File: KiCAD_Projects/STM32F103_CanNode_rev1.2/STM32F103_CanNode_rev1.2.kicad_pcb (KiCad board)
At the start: 2 copper layers, 35 x 50 mm, 77 parts, among them P1 CONN_01X04, P10 CONN_01X04, P11 CONN_01X04, P12 CONN_01X02, P2 CONN_01X04, P3 CONN_01X08, P4 CONN_01X08, P5 CONN_01X06, P6 CONN_01X02, P7 CONN_01X08, P8 CONN_01X04, P9 CONN_01X04, SW1 SW_PUSH, SW2 SW_PUSH, U1 STM32F103_48, U2 AOZ1280, U3 MAX3051, U4 NCP1117ST50T3G, U5 TBD62083A, X2 CRYSTAL

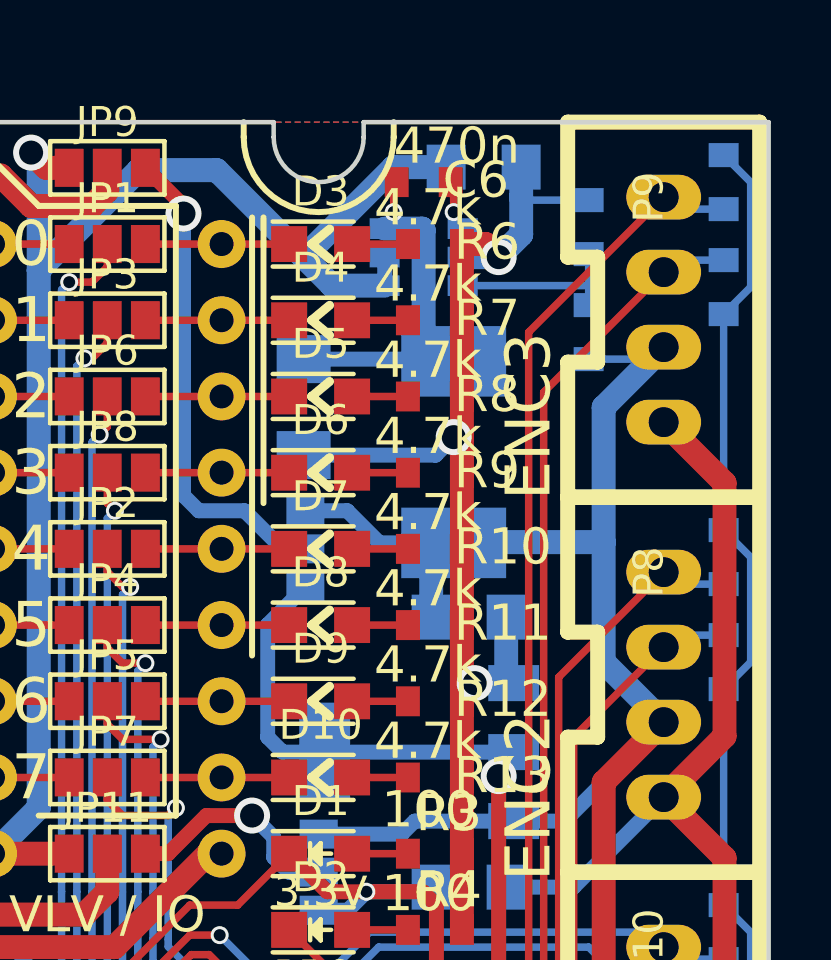
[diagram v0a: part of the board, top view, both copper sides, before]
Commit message: セルチェッカー作った｡電源基板ver1.1作った｡ぶっさしMDいじった｡DCDCいじりだした｡
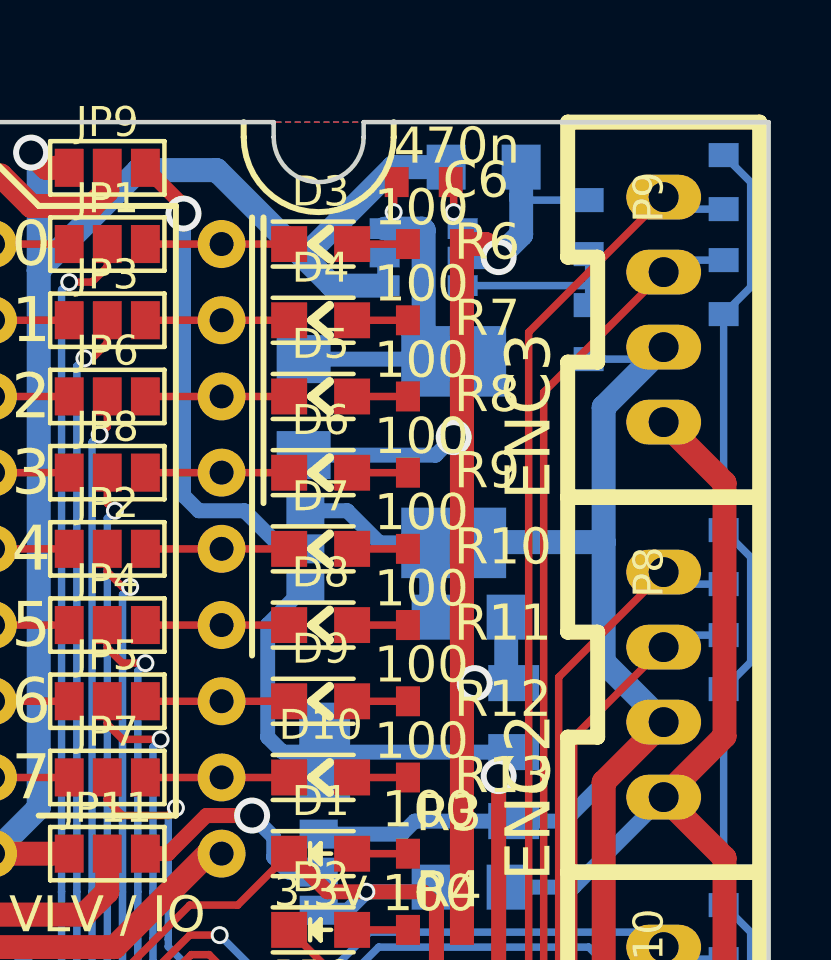
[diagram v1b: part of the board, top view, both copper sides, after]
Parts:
- R10, R11, R12, R13, R6, R7, R8, R9: value 4.7k -> 100
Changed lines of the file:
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@@
     (links 193)
     (no_connects 0)
-    (area -0.075001 -0.075001 35.075001 50.075001)
+    (area -3.509333 -2.533334 35.150001 52.533333)
     (thickness 1.6)
     (drawings 50)
@@
       (effects (font (size 1.2065 1.2065) (thickness 0.1016)) (justify left bottom))
     )
-    (fp_text value 4.7k (at 2.032 0.508 180) (layer F.SilkS)
+    (fp_text value 100 (at 2.032 0.508 180) (layer F.SilkS)
       (effects (font (size 1.2065 1.2065) (thickness 0.1016)) (justify left bottom))
     )
@@
       (effects (font (size 1.2065 1.2065) (thickness 0.1016)) (justify left bottom))
     )
-    (fp_text value 4.7k (at 2.032 0.508 180) (layer F.SilkS)
+    (fp_text value 100 (at 2.032 0.508 180) (layer F.SilkS)
       (effects (font (size 1.2065 1.2065) (thickness 0.1016)) (justify left bottom))
     )
@@
       (effects (font (size 1.2065 1.2065) (thickness 0.1016)) (justify left bottom))
     )
-    (fp_text value 4.7k (at 2.032 0.508 180) (layer F.SilkS)
+    (fp_text value 100 (at 2.032 0.508 180) (layer F.SilkS)
       (effects (font (size 1.2065 1.2065) (thickness 0.1016)) (justify left bottom))
     )
@@
       (effects (font (size 1.2065 1.2065) (thickness 0.1016)) (justify left bottom))
     )
-    (fp_text value 4.7k (at 2.032 0.508 180) (layer F.SilkS)
+    (fp_text value 100 (at 2.032 0.508 180) (layer F.SilkS)
       (effects (font (size 1.2065 1.2065) (thickness 0.1016)) (justify left bottom))
     )
@@
       (effects (font (size 1.2065 1.2065) (thickness 0.1016)) (justify left bottom))
     )
-    (fp_text value 4.7k (at 2.032 0.508 180) (layer F.SilkS)
+    (fp_text value 100 (at 2.032 0.508 180) (layer F.SilkS)
       (effects (font (size 1.2065 1.2065) (thickness 0.1016)) (justify left bottom))
     )
@@
       (effects (font (size 1.2065 1.2065) (thickness 0.1016)) (justify left bottom))
     )
-    (fp_text value 4.7k (at 2.032 0.508 180) (layer F.SilkS)
+    (fp_text value 100 (at 2.032 0.508 180) (layer F.SilkS)
       (effects (font (size 1.2065 1.2065) (thickness 0.1016)) (justify left bottom))
     )
@@
       (effects (font (size 1.2065 1.2065) (thickness 0.1016)) (justify left bottom))
     )
-    (fp_text value 4.7k (at 2.032 0.508 180) (layer F.SilkS)
+    (fp_text value 100 (at 2.032 0.508 180) (layer F.SilkS)
       (effects (font (size 1.2065 1.2065) (thickness 0.1016)) (justify left bottom))
     )
@@
       (effects (font (size 1.2065 1.2065) (thickness 0.1016)) (justify left bottom))
     )
-    (fp_text value 4.7k (at 2.032 0.508 180) (layer F.SilkS)
+    (fp_text value 100 (at 2.032 0.508 180) (layer F.SilkS)
       (effects (font (size 1.2065 1.2065) (thickness 0.1016)) (justify left bottom))
     )
@@
       (effects (font (size 1.2065 1.2065) (thickness 0.1016)) (justify left bottom mirror))
     )
-    (fp_text value 0.1u (at 0.88 -0.67) (layer B.SilkS)
+    (fp_text value 0.1u (at 2.88 4.33) (layer B.SilkS)
       (effects (font (size 1.2065 1.2065) (thickness 0.1016)) (justify left bottom mirror))
     )
@@
       (effects (font (size 1.2065 1.2065) (thickness 0.1016)) (justify left bottom mirror))
     )
-    (fp_text value 4.7k (at -1.5 1 270) (layer B.SilkS)
+    (fp_text value 4.7k (at -0.5 0.5 360) (layer B.SilkS)
       (effects (font (size 1.2065 1.2065) (thickness 0.1016)) (justify left bottom mirror))
     )
@@
       (effects (font (size 1.2065 1.2065) (thickness 0.1016)) (justify left bottom mirror))
     )
-    (fp_text value 4.7k (at -0.5 0.5 180) (layer B.SilkS)
+    (fp_text value 4.7k (at -1.5 1 270) (layer B.SilkS)
       (effects (font (size 1.2065 1.2065) (thickness 0.1016)) (justify left bottom mirror))
     )
@@
   (segment (start 10.668 4.932) (end 10.668 22.86) (width 0.8) (layer B.Cu) (net 3))
   (segment (start 11.684 24.384) (end 9.144 24.384) (width 0.8) (layer F.Cu) (net 3))
-  (segment (start 20.045584 38.356245) (end 21.5 39.810661) (width 0.25) (layer F.Cu) (net 4) (status 400000))
-  (segment (start 22.5 42.3) (end 22.5 44.3) (width 0.25) (layer B.Cu) (net 4) (status 800000))
+  (segment (start 20.045584 38.356245) (end 21.5 39.810661) (width 0.25) (layer F.Cu) (net 4))
+  (segment (start 22.5 42.3) (end 22.5 44.3) (width 0.25) (layer B.Cu) (net 4))
   (via (at 22.5 42.3) (size 0.6) (drill 0.4) (layers F.Cu B.Cu) (net 4))
   (segment (start 21.5 41.3) (end 22.5 42.3) (width 0.25) (layer F.Cu) (net 4))
@@
   (segment (start 22.3 44.5) (end 22.5 44.3) (width 0.25) (layer B.Cu) (net 4))
   (segment (start 22.2 45) (end 22.5 45.3) (width 0.25) (layer B.Cu) (net 4))
-  (segment (start 20.399138 38.002691) (end 22 39.603553) (width 0.25) (layer F.Cu) (net 5) (status 400000))
+  (segment (start 20.399138 38.002691) (end 22 39.603553) (width 0.25) (layer F.Cu) (net 5))
   (via (at 22.5 41) (size 0.6) (drill 0.4) (layers F.Cu B.Cu) (net 5))
   (segment (start 22 40.5) (end 22.5 41) (width 0.25) (layer F.Cu) (net 5))
   (segment (start 22 39.603553) (end 22 40.5) (width 0.25) (layer F.Cu) (net 5))
-  (segment (start 22.5 39.7) (end 22.5 41) (width 0.25) (layer B.Cu) (net 5) (status 400000))
-  (segment (start 21.5 42) (end 19.9 42) (width 0.25) (layer B.Cu) (net 5) (status 800000))
+  (segment (start 22.5 39.7) (end 22.5 41) (width 0.25) (layer B.Cu) (net 5))
+  (segment (start 21.5 42) (end 19.9 42) (width 0.25) (layer B.Cu) (net 5))
   (segment (start 22.5 41) (end 21.5 42) (width 0.25) (layer B.Cu) (net 5))
   (segment (start 21.9 39.8) (end 21.9 40.1) (width 0.25) (layer B.Cu) (net 5))
@@
   (segment (start 4.064 11.684) (end 4.064 9.144) (width 0.8) (layer F.Cu) (net 44))
   (segment (start 25.1 36.5) (end 28.8 36.5) (width 0.25) (layer B.Cu) (net 45))
-  (segment (start 30.9 38.6) (end 33.5 38.6) (width 0.25) (layer B.Cu) (net 45) (status 800000))
+  (segment (start 30.9 38.6) (end 33.5 38.6) (width 0.25) (layer B.Cu) (net 45))
   (segment (start 28.8 36.5) (end 30.9 38.6) (width 0.25) (layer B.Cu) (net 45))
   (segment (start 25.4 30.2) (end 23.925998 28.725998) (width 0.5) (layer F.Cu) (net 45))
@@
   (segment (start 29 4.4) (end 29 5.5) (width 0.25) (layer B.Cu) (net 68))
   (segment (start 29 5.5) (end 29 6.1) (width 0.25) (layer B.Cu) (net 68))
-  (segment (start 28.04 40) (end 28.04 38.54) (width 0.25) (layer B.Cu) (net 69) (status 400000))
+  (segment (start 28.04 40) (end 28.04 38.54) (width 0.25) (layer B.Cu) (net 69))
   (segment (start 27.6 38.1) (end 20.7 38.1) (width 0.25) (layer B.Cu) (net 69))
   (segment (start 28.04 38.54) (end 27.6 38.1) (width 0.25) (layer B.Cu) (net 69))
-  (segment (start 28.04 40) (end 28.04 39.54) (width 0.25) (layer B.Cu) (net 69) (status C00000))
+  (segment (start 28.04 40) (end 28.04 39.54) (width 0.25) (layer B.Cu) (net 69))
   (segment (start 19.8 40.5) (end 19.8 39) (width 0.25) (layer B.Cu) (net 69))
   (segment (start 19.8 40.231981) (end 19.8 40.5) (width 0.25) (layer F.Cu) (net 69))
@@
   (segment (start 19.8 39) (end 20.7 38.1) (width 0.25) (layer B.Cu) (net 69))
   (segment (start 19.338478 39.063351) (end 20.5 40.224873) (width 0.25) (layer F.Cu) (net 70))
-  (segment (start 22.7 43.5) (end 25.7 43.5) (width 0.25) (layer F.Cu) (net 70) (status 800000))
+  (segment (start 22.7 43.5) (end 25.7 43.5) (width 0.25) (layer F.Cu) (net 70))
   (segment (start 20.5 41.3) (end 22.7 43.5) (width 0.25) (layer F.Cu) (net 70))
   (segment (start 20.5 40.224873) (end 20.5 41.3) (width 0.25) (layer F.Cu) (net 70))
